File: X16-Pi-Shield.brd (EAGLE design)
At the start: 81.3 x 74.3 mm, 36 parts, among them J3 CONN_DF13-4P-1.25DSA, J4 HTST-110-04-L-D-RA, J5 BM04B-GHS-TBT, U1 INA260AIPW, U2 AZ1117IH-3.3TRG1

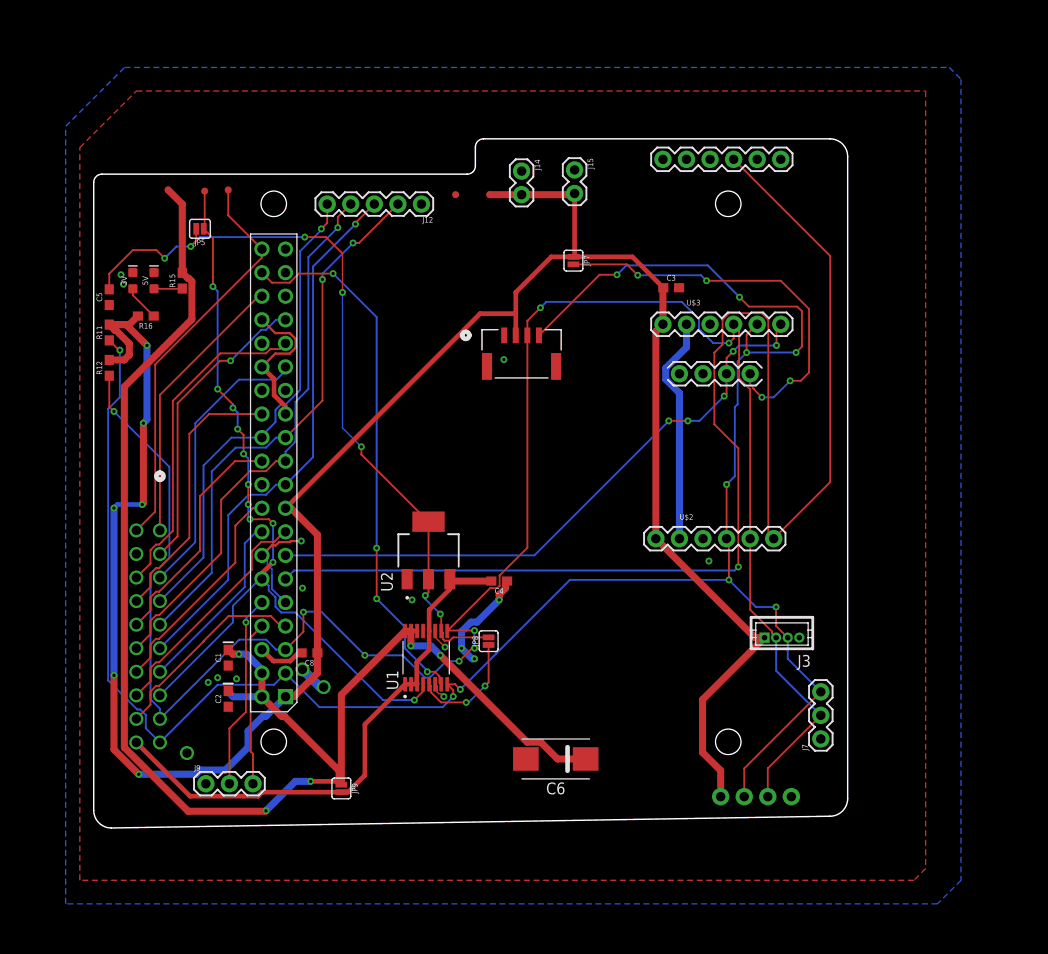
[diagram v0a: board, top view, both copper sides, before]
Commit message: remade the board
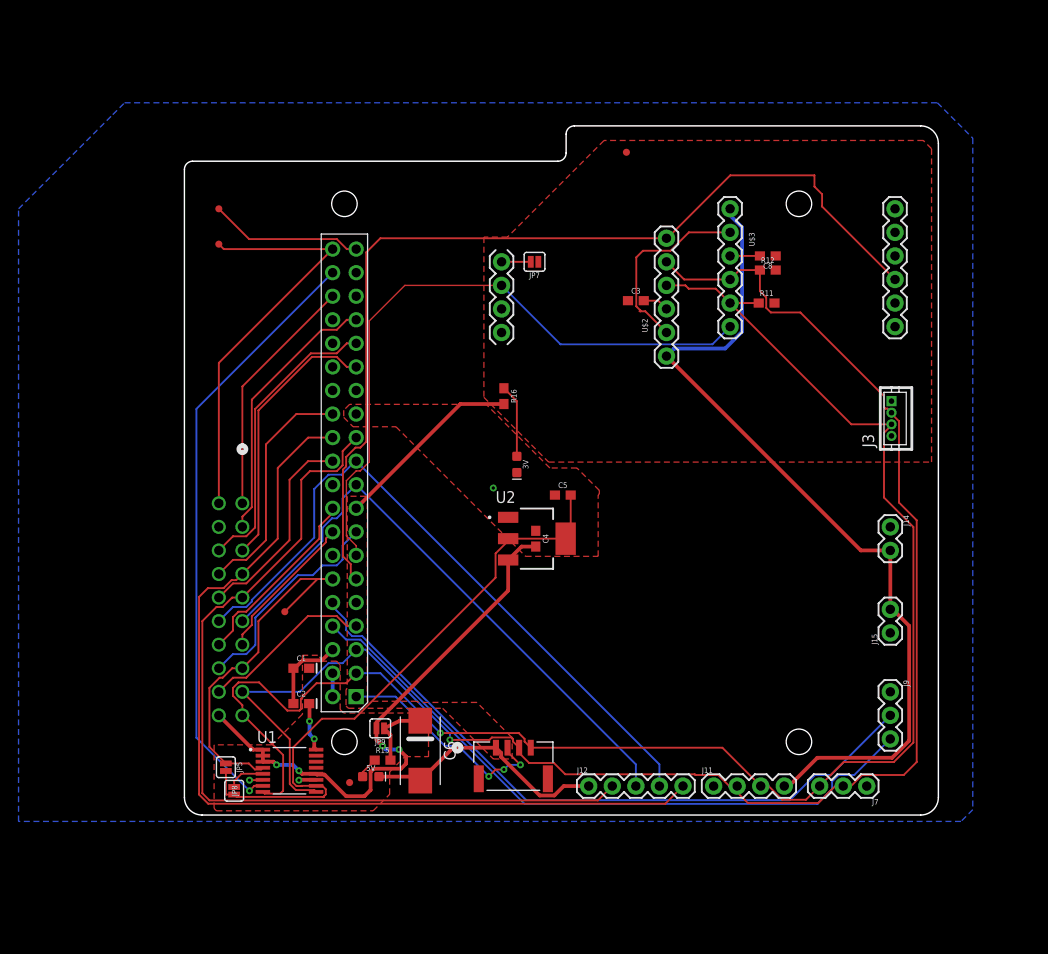
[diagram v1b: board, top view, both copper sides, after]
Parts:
- moved J9 74.4 mm to (74.9, 12.7), turned to 270 degrees
- moved R12 71.8 mm to (61.7, 58.2), turned to 0 degrees
- moved R11 70.9 mm to (61.6, 54.6), turned to 0 degrees
- moved TP7 66.8 mm to (16.6, 2.92)
- moved C8 65.4 mm to (61.7, 59.7)
- moved J12 65.3 mm to (42.4, 2.54), turned to 0 degrees
- moved J15 60.4 mm to (74.9, 19.1), turned to 90 degrees
- moved 5V 58.4 mm to (18.9, 3.56), turned to 0 degrees
- moved JP5 58.1 mm to (3.30, 4.57), turned to 270 degrees
- moved R15 56.0 mm to (20.2, 5.33), turned to 0 degrees
- moved J14 55.2 mm to (74.9, 30.5)
- moved C5 53.3 mm to (39.6, 33.9), turned to 0 degrees
- moved TP5 46.2 mm to (9.65, 21.3)
- moved 3V 45.9 mm to (34.7, 37.2), turned to 270 degrees
- moved J5 44.5 mm to (34.3, 4.70)
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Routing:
- net 5V: track 162.4 -> 15.6 mm, vias 5 -> 2
- net 3V3: track 247.1 -> 137.6 mm, vias 6 -> 3
- net SDA: track 225.4 -> 170.9 mm, vias 10 -> 1
- net TX: track 17.6 -> 71.5 mm
- net RX: track 21.0 -> 73.6 mm, vias 1 -> 0
- net IMU_RESET: track 154.5 -> 103.7 mm, vias 1 -> 0
- net SA1: track 88.7 -> 39.9 mm, vias 11 -> 0
- net CS: track 52.6 -> 100.7 mm, vias 1 -> 0
- net N$17: track 43.6 -> 3.15 mm, vias 4 -> 0
- net SCL: track 213.0 -> 173.6 mm, vias 8 -> 1
- net CLK: track 58.9 -> 93.1 mm, vias 2 -> 0
- net VS: track 83.5 -> 67.1 mm, vias 7 -> 0
- net MISO: track 59.3 -> 73.7 mm, vias 1 -> 0
- net GND: track 50.8 -> 61.9 mm, vias 17 -> 3
- net N$3: track 12.5 -> 4.06 mm, vias 2 -> 0
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- added copper zone on layer 1, net 3V3
- added copper zone on layer 1, net 5V
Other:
- outline, holes or cut-outs redrawn

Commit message: remade board
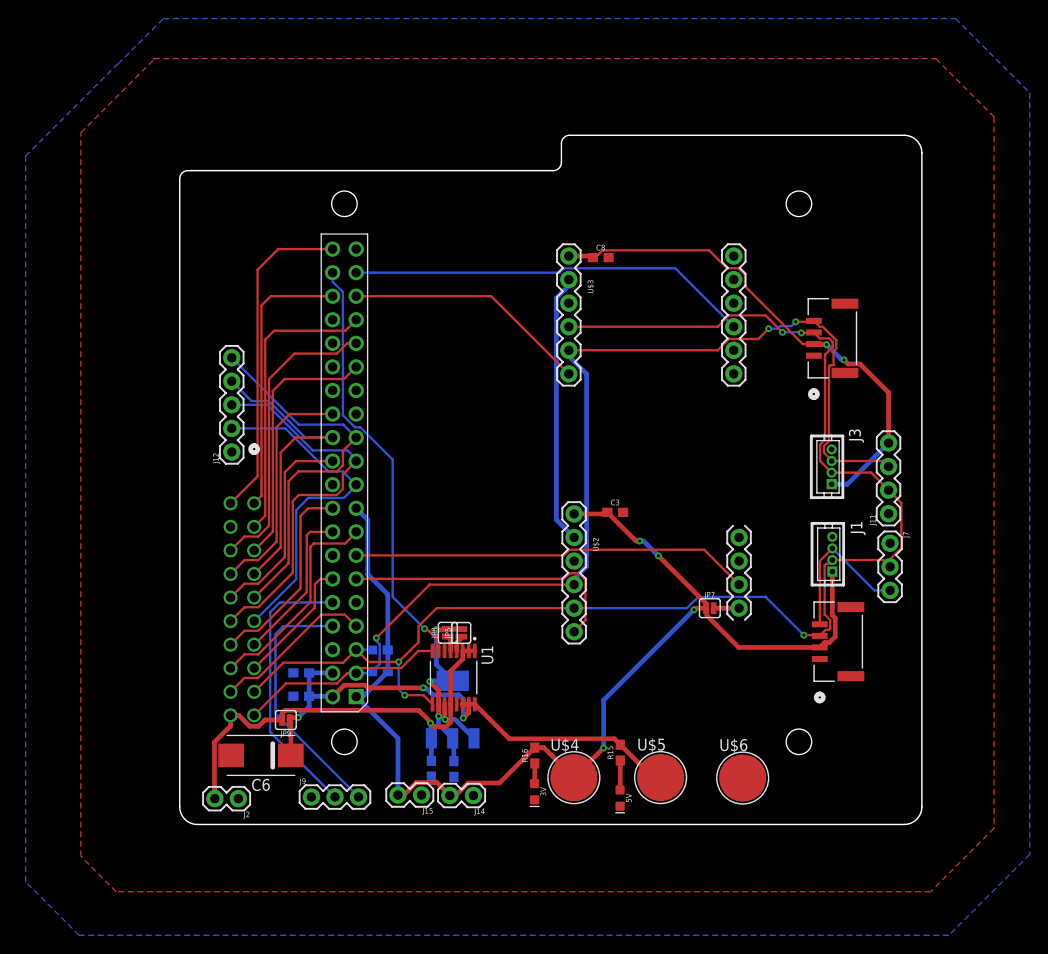
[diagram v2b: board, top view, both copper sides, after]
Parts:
- removed TP4, TP5, TP6, TP7, TP8: TEST-POINT3, SparkFun-Connectors:PAD.03X.03
- added J1: CONN_DF13-4P-1.25DSA, X16-Pi-Shield:DF13-4P-1.25DSA
- added J2: (no value), SparkFun-Connectors:1X02
- added J6: BM04B-GHS-TBT, X16-Pi-Shield:CONN_BM04B-GHS-TBT_JST
- added U$4, U$5, U$6: TESTPOINT_5.04MM, X16-ExtraComponents:TESTPOINT_5.04MM
- moved J9 63.4 mm to (12.5, 1.36), turned to 0 degrees
- moved R12 58.5 mm to (19.9, 17.2), flipped to the bottom, turned to 180 degrees
- moved R11 57.6 mm to (19.9, 14.9), flipped to the bottom, turned to 180 degrees
- moved J5 57.5 mm to (68.7, 50.8), turned to 90 degrees
- moved J15 53.5 mm to (24.4, 1.57), turned to 180 degrees
- moved J14 53.5 mm to (30.0, 1.52), turned to 180 degrees
- moved J12 52.7 mm to (3.94, 38.6), turned to 90 degrees
- moved JP7 41.8 mm to (55.5, 21.7), turned to 0 degrees
- moved R16 38.9 mm to (36.6, 5.83), turned to 90 degrees
- moved 3V 35.3 mm to (36.6, 1.93)
- moved J11 34.9 mm to (74.7, 31.9), turned to 90 degrees
- moved C5 31.8 mm to (27.9, 4.38), flipped to the bottom, turned to 90 degrees
- moved JP5 29.2 mm to (28.7, 19.1), turned to 90 degrees
- moved JP8 28.6 mm to (27.2, 19.1), turned to 90 degrees
- moved C4 27.2 mm to (25.5, 4.41), flipped to the bottom, turned to 90 degrees
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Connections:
- new net IMU_INT_2: U$1.35, U$3.INT
- new net IMU_RESET_2: U$1.37, U$3.RST
- new net N$1: JP5.1, U1.4
- net 3V3: now also J1.1, J6.2, U$4.TP; no longer TP6.1
- net 5V: now also U$5.TP; no longer TP7.1
- net 5V_EXT: now also J2.2
- net CLK: now also J12.5; no longer J12.2
- net CS: now also J12.4; no longer J12.5
- net GND: now also J1.4, J2.1, J6.1, U$6.TP; no longer TP8.1
- net IMU_INT: no longer U$3.INT
- net IMU_RESET: no longer U$3.RST
- net MISO: now also J12.3; no longer J12.4
- net MOSI: now also J12.2; no longer J12.3
- net SA0: no longer TP4.1
- net SA1: no longer JP5.1, TP5.1, U1.4
- net SCL: now also J1.2, J6.3
- net SDA: now also J1.3, J6.4
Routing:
- net IMU_RESET: track 103.7 -> 31.4 mm
- net CS: track 100.7 -> 33.9 mm
- net GND: track 61.9 -> 5.63 mm, vias 3 -> 1
- net CLK: track 93.1 -> 41.2 mm
- net VS: track 67.1 -> 21.1 mm, vias 0 -> 3
- net 3V3: track 137.6 -> 182.4 mm, vias 3 -> 6
- net TX: track 71.5 -> 27.8 mm
- net RX: track 73.6 -> 30.0 mm
- net IMU_RESET_2: track 0.00 -> 43.5 mm
- net 5V: track 15.6 -> 59.0 mm, vias 2 -> 3
- net MISO: track 73.7 -> 42.2 mm
- net IMU_INT: track 70.9 -> 43.1 mm
- net MOSI: track 65.1 -> 37.4 mm
- net IMU_INT_2: track 0.00 -> 26.4 mm
- net SA1: track 39.9 -> 13.9 mm
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- removed copper zone on layer 1, net 3V3
- removed copper zone on layer 1, net 5V
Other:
- board size 81.3 x 74.3 mm -> 80 x 74.3 mm
